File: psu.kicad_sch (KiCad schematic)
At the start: 7 parts, among them Q6 PMOS, SW1 SW_SPDT, U2 AP7380-33Y-13

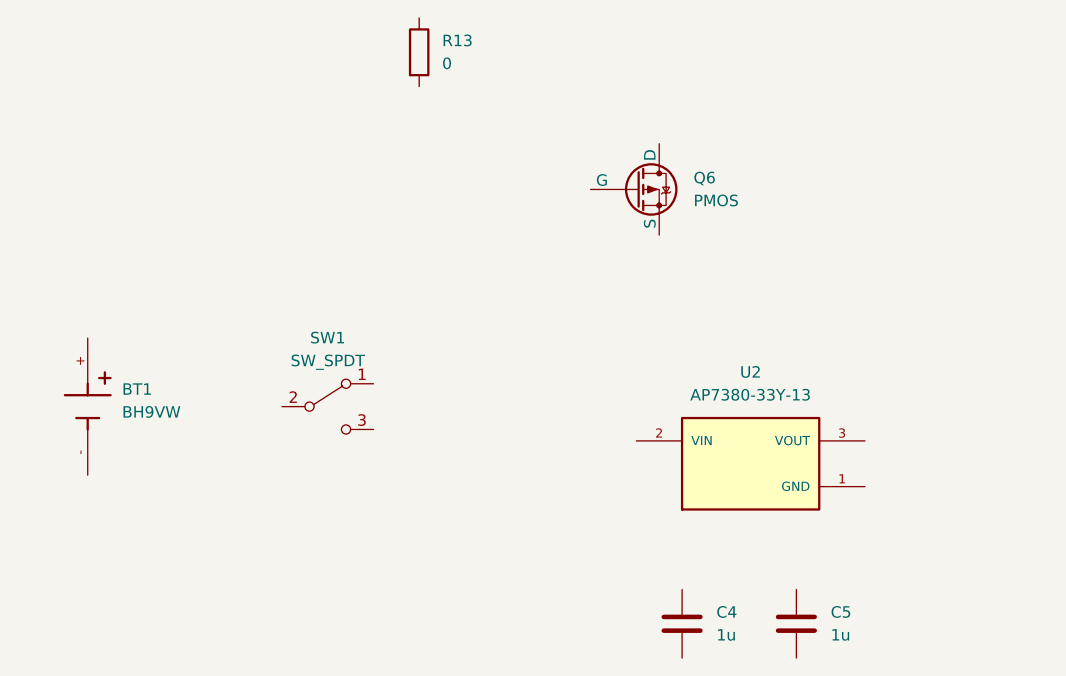
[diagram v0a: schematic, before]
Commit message: sym
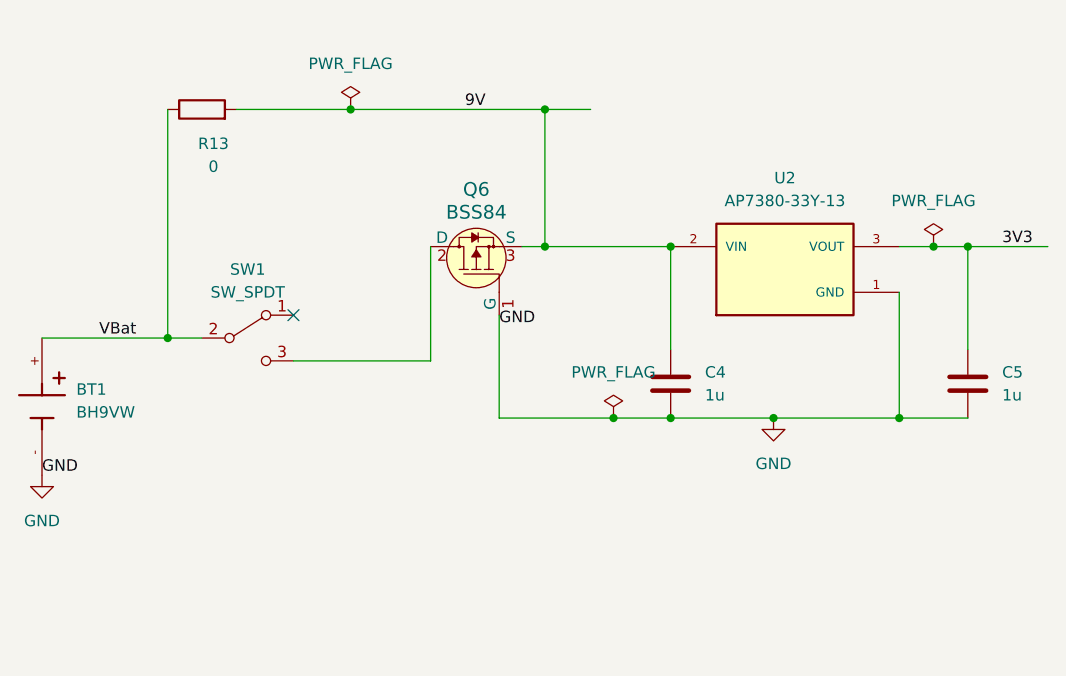
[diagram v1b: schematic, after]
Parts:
- removed Q6: PMOS, symbol Simulation_SPICE:PMOS
- added Q6: BSS84, digikey-footprints:SOT-23-3, symbol dk_Transistors-FETs-MOSFETs-Single:BSS84
- BT1: footprint BAT_BH9VW -> BH9VW:BAT_BH9VW_SMD
- C4, C5: footprint (none) -> Capacitor_SMD:C_0603_1608Metric
- R13: footprint (none) -> Resistor_SMD:R_0805_2012Metric
- U2: footprint VREG_AP7380-33Y-13 -> AP7380-33Y-13:VREG_AP7380-33Y-13
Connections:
- net 9V: now reaches C4.1
- net 9V: now also R13.2, U2.2 (VIN), Q6.3 (S)
- net GND: now reaches C4.2
- net GND: now also BT1.-, C5.2, U2.1 (GND), Q6.1 (G)
- net VBat: now reaches R13.1
- net VBat: now also BT1.+, SW1.2 (B)
- net at SW1.3 (C): now also Q6.2 (D)
- net 3V3: now reaches U2.3 (VOUT)
- net 3V3: now also C5.1
- no-connect marks 0 -> 1
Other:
- moved on the sheet: BT1, C4, C5, R13, SW1, U2
